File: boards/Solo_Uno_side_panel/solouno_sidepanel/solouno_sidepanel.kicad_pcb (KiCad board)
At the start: 2 copper layers, 29 x 80 mm, 11 parts, among them CN1 CAN Front, CN2 CAN Back

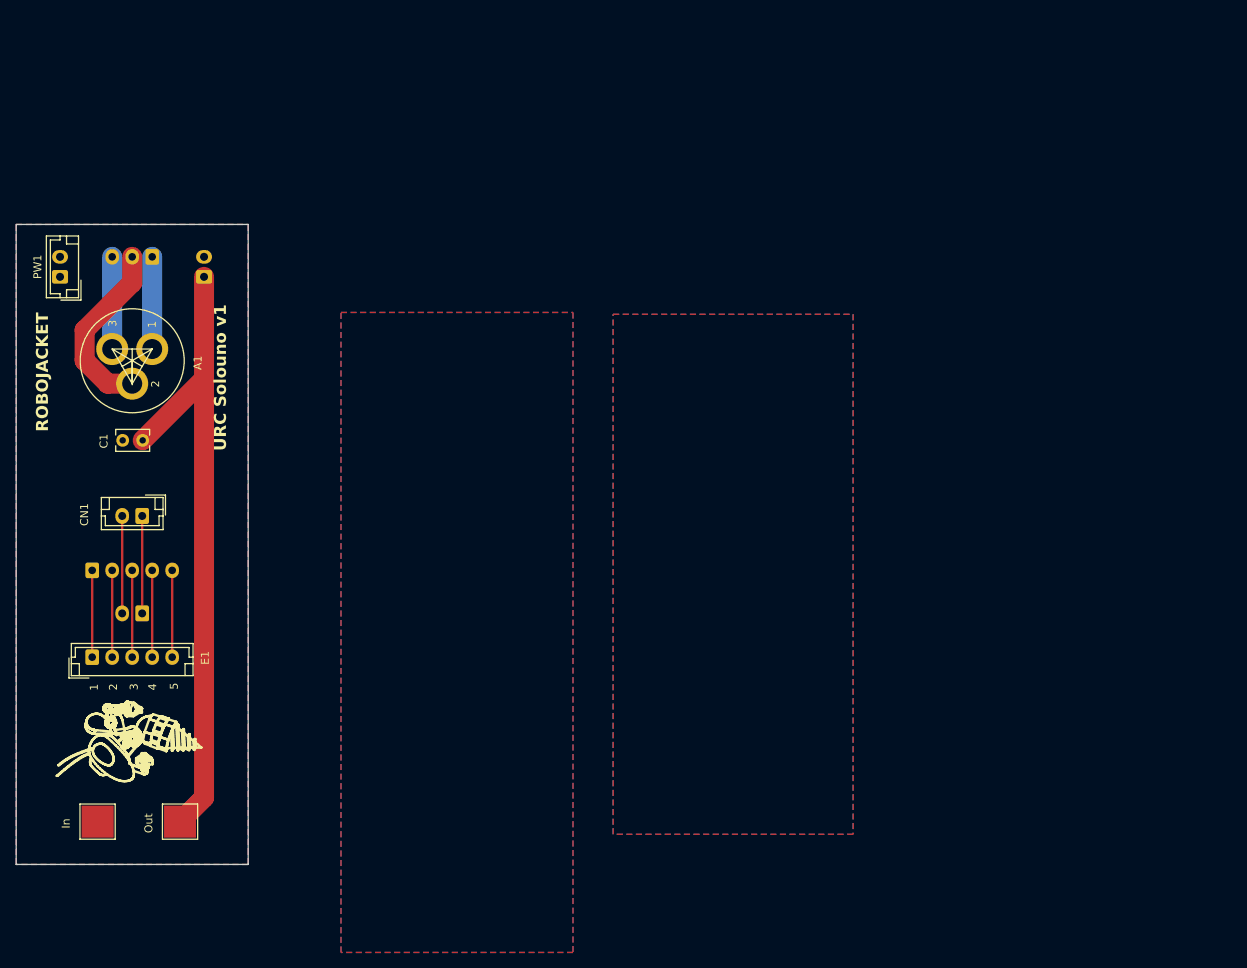
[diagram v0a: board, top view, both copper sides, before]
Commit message: solouno update
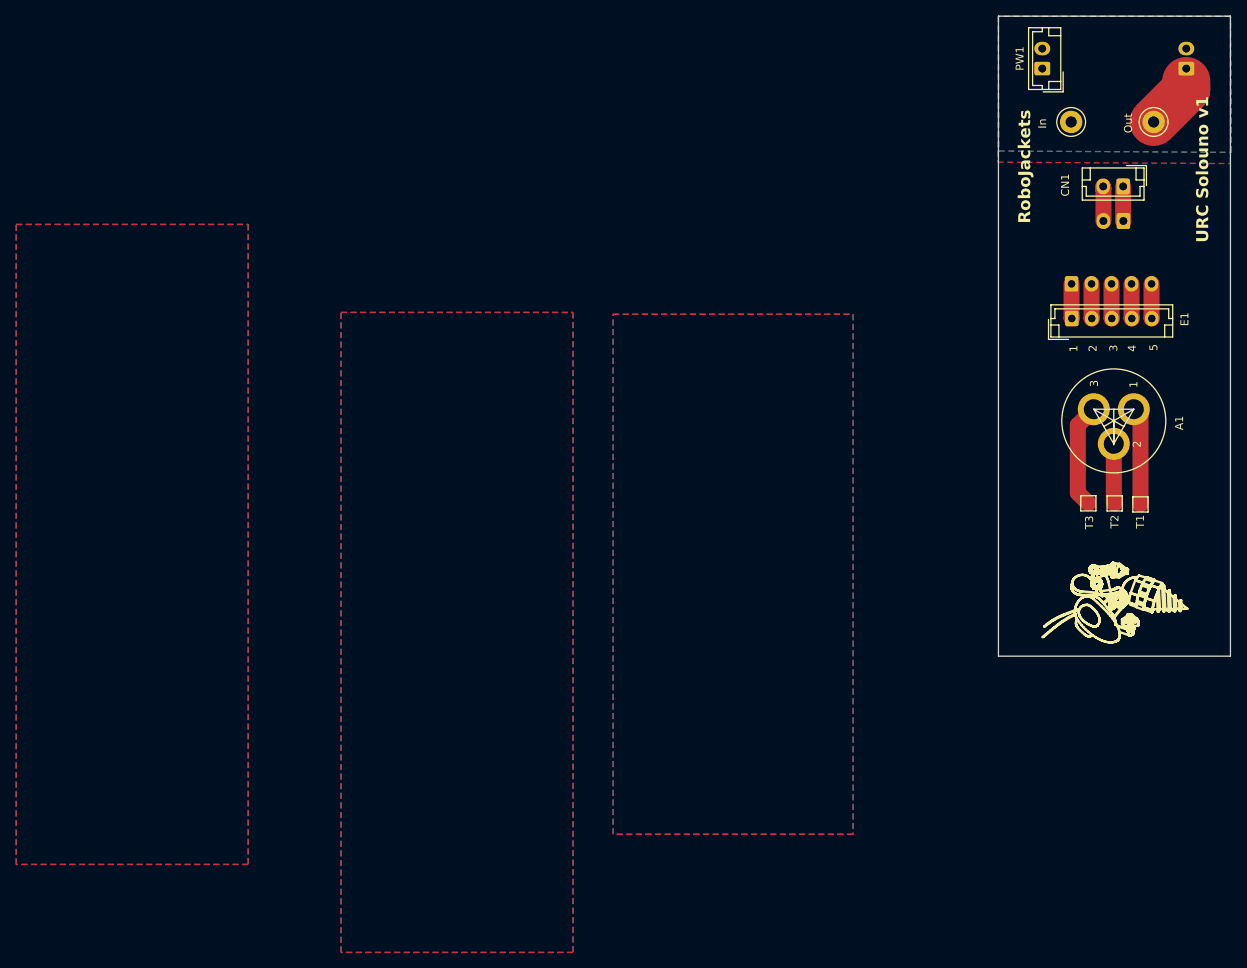
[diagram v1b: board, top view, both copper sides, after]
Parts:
- removed A2: Aviation Pin, Connector_JST:JST_EH_B3B-EH-A_1x03_P2.50mm_Vertical
- removed C1: 3.3uF, Capacitor_THT:C_Rect_L4.0mm_W2.5mm_P2.50mm
- added T1: Test1, TestPoint:TestPoint_Pad_1.5x1.5mm, F.Cu at (193.0, 124.6)
- added T2: Test2, TestPoint:TestPoint_Pad_1.5x1.5mm, F.Cu at (189.8, 124.5)
- added T3: Test3, TestPoint:TestPoint_Pad_1.5x1.5mm, F.Cu at (186.5, 124.4)
- S1, S2: footprint TestPoint:TestPoint_Pad_4.0x4.0mm -> TestPoint:TestPoint_Loop_D3.50mm_Drill1.4mm_Beaded
- moved S1 149.9 mm to (184.4, 76.8)
- moved S2 149.9 mm to (194.7, 76.8)
- moved CN2 132.1 mm to (190.9, 89.2)
- moved E1 129.6 mm to (184.5, 101.3)
- moved CN1 129.4 mm to (190.9, 84.8)
- moved E2 127.6 mm to (184.4, 97.0)
- moved PW2 125.5 mm to (198.8, 70.1)
- moved PW1 125.5 mm to (180.8, 70.1)
- moved A1 122.9 mm to (189.7, 114.1)
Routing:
- net Net-(PW2-Pin_1): track 80.2 -> 6.81 mm
- net Net-(A1-Pad2): track 22.6 -> 7.83 mm
- net Net-(CN1-Pin_2): track 12.2 -> 4.33 mm
- net Net-(CN1-Pin_1): track 12.2 -> 4.33 mm
- net Net-(E1-Pin_5): track 10.8 -> 4.34 mm
- net Net-(E1-Pin_4): track 10.8 -> 4.34 mm
- net Net-(E1-Pin_3): track 10.8 -> 4.34 mm
- net Net-(E1-Pin_2): track 10.8 -> 4.34 mm
- net Net-(E1-Pin_1): track 10.8 -> 4.34 mm
- net Net-(A1-Pad3): track 11.5 -> 13.1 mm
- net Net-(A1-Pad1): track 11.5 -> 12.2 mm
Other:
- board text added: "RoboJackets"
- board text removed: "ROBOJACKET"
